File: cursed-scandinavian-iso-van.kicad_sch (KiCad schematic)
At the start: 105 parts, among them J1 Conn_01x04, SW1 SW_Push, U1 ATmega32U4-A, Y1 16MHz

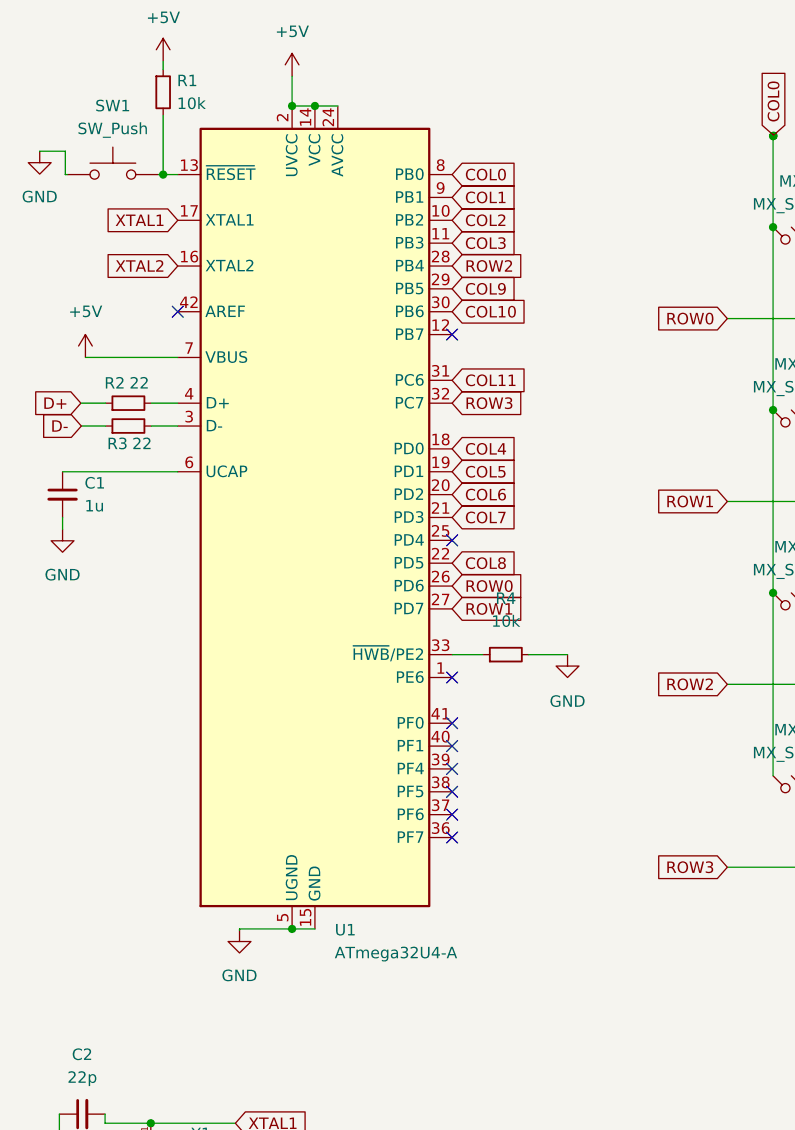
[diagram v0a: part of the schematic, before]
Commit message: second attempt
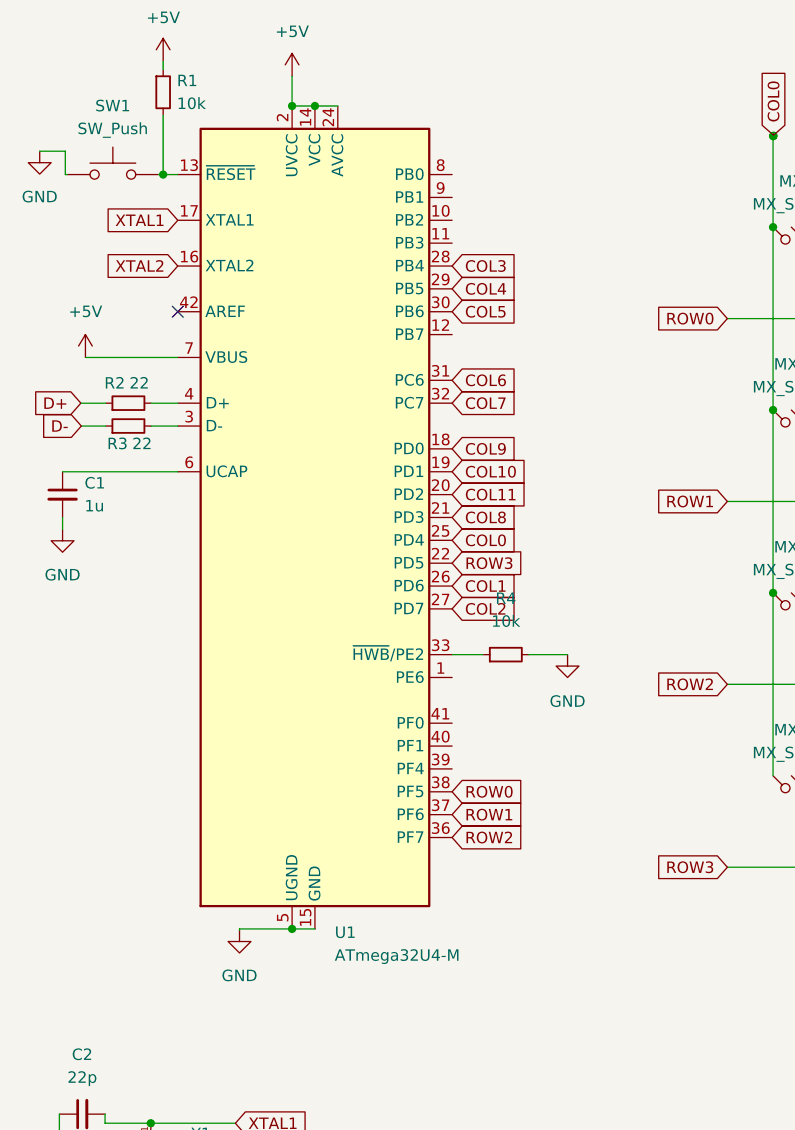
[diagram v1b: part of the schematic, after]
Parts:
- removed U1: ATmega32U4-A, Package_QFP:TQFP-44_10x10mm_P0.8mm, symbol MCU_Microchip_ATmega:ATmega32U4-A
- added U1: ATmega32U4-M, Package_DFN_QFN:QFN-44-1EP_7x7mm_P0.5mm_EP5.2x5.2mm, symbol MCU_Microchip_ATmega:ATmega32U4-M
- C1, C2, C3, C4, C5, C6, C7: footprint Capacitor_SMD:C_0805_2012Metric -> Capacitor_SMD:C_0402_1005Metric
- R1, R2, R3, R4: footprint Resistor_SMD:R_0805_2012Metric -> Resistor_SMD:R_0402_1005Metric
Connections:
- net +5V: now also U1.14 (VCC), U1.2 (UVCC), U1.24 (AVCC), U1.34 (VCC), U1.44 (AVCC), U1.7 (VBUS)
- net COL0: now also U1.25 (PD4)
- net COL1: now also U1.26 (PD6)
- net COL10: now also U1.19 (PD1)
- net COL11: now also U1.20 (PD2)
- net COL2: now also U1.27 (PD7)
- net COL3: now also U1.28 (PB4)
- net COL4: now also U1.29 (PB5)
- net COL5: now also U1.30 (PB6)
- net COL6: now also U1.31 (PC6)
- net COL7: now also U1.32 (PC7)
- net COL8: now also U1.21 (PD3)
- net COL9: now also U1.18 (PD0)
- net GND: now also U1.15 (GND), U1.23 (GND), U1.35 (GND), U1.43 (GND), U1.45 (GND), U1.5 (UGND)
- net ROW0: now also U1.38 (PF5)
- net ROW1: now also U1.37 (PF6)
- net ROW2: now also U1.36 (PF7)
- net ROW3: now also U1.22 (PD5)
- net XTAL1: now also U1.17 (XTAL1)
- net XTAL2: now also U1.16 (XTAL2)
- net at R1.2, SW1.1: now also U1.13 (~{RESET})
- net at R3.2: now also U1.3 (D-)
- net at R4.1: now also U1.33 (~{HWB}/PE2)
- net at R2.2: now also U1.4 (D+)
- net at C1.1: now also U1.6 (UCAP)
- no-connect marks 10 -> 1

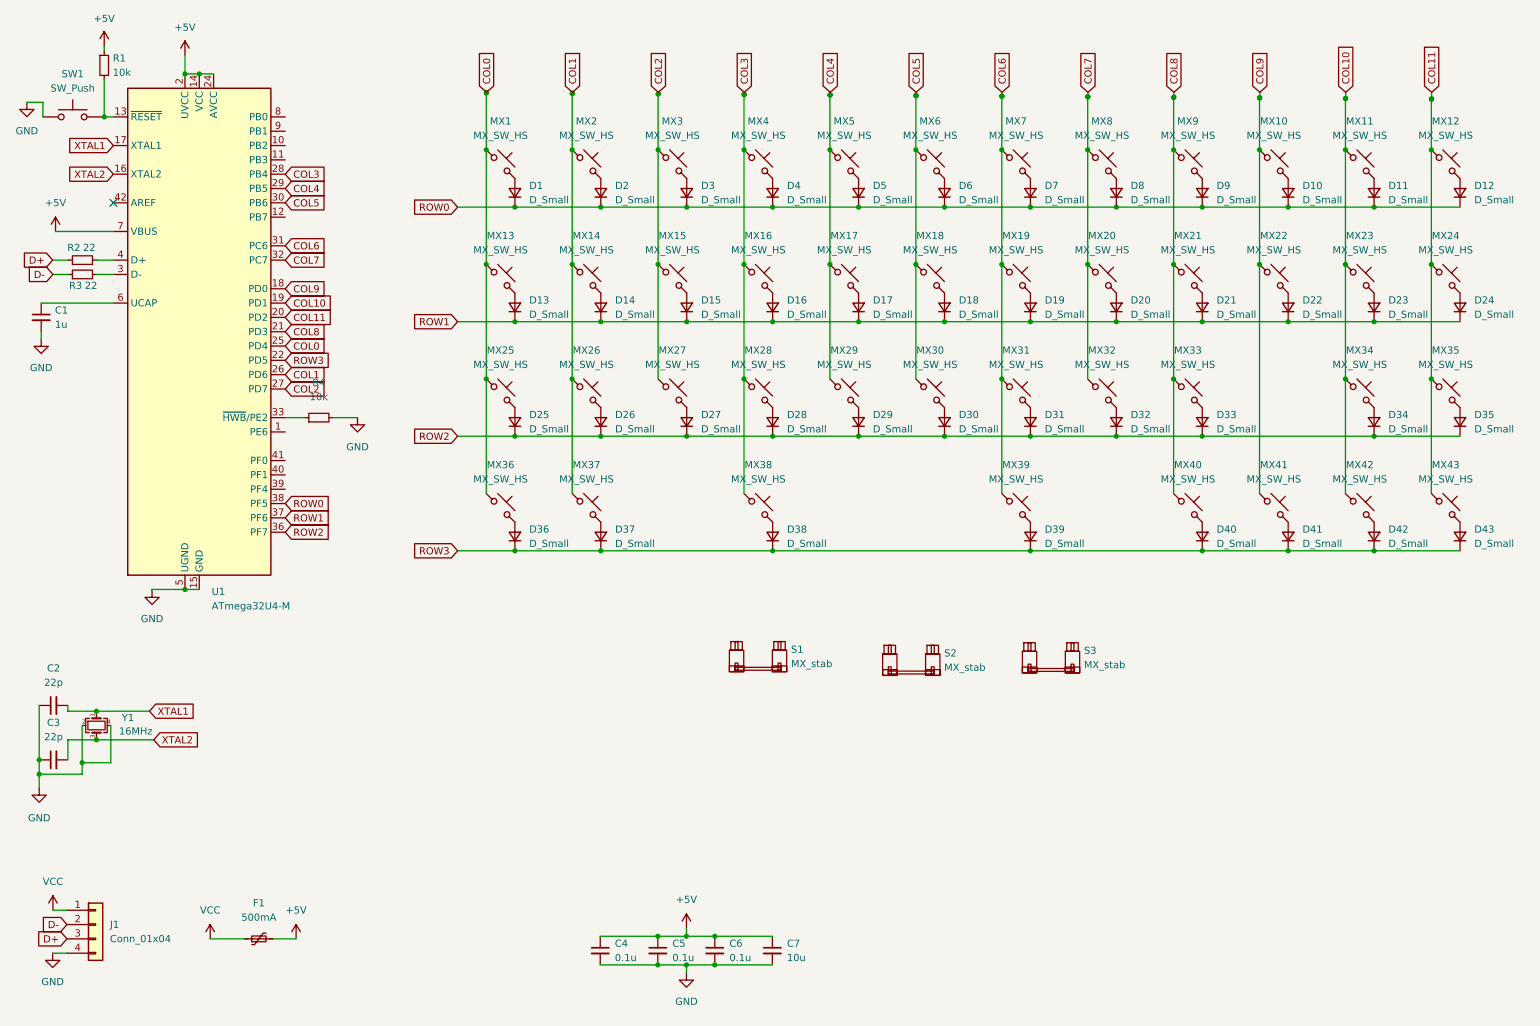
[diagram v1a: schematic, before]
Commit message: maybe
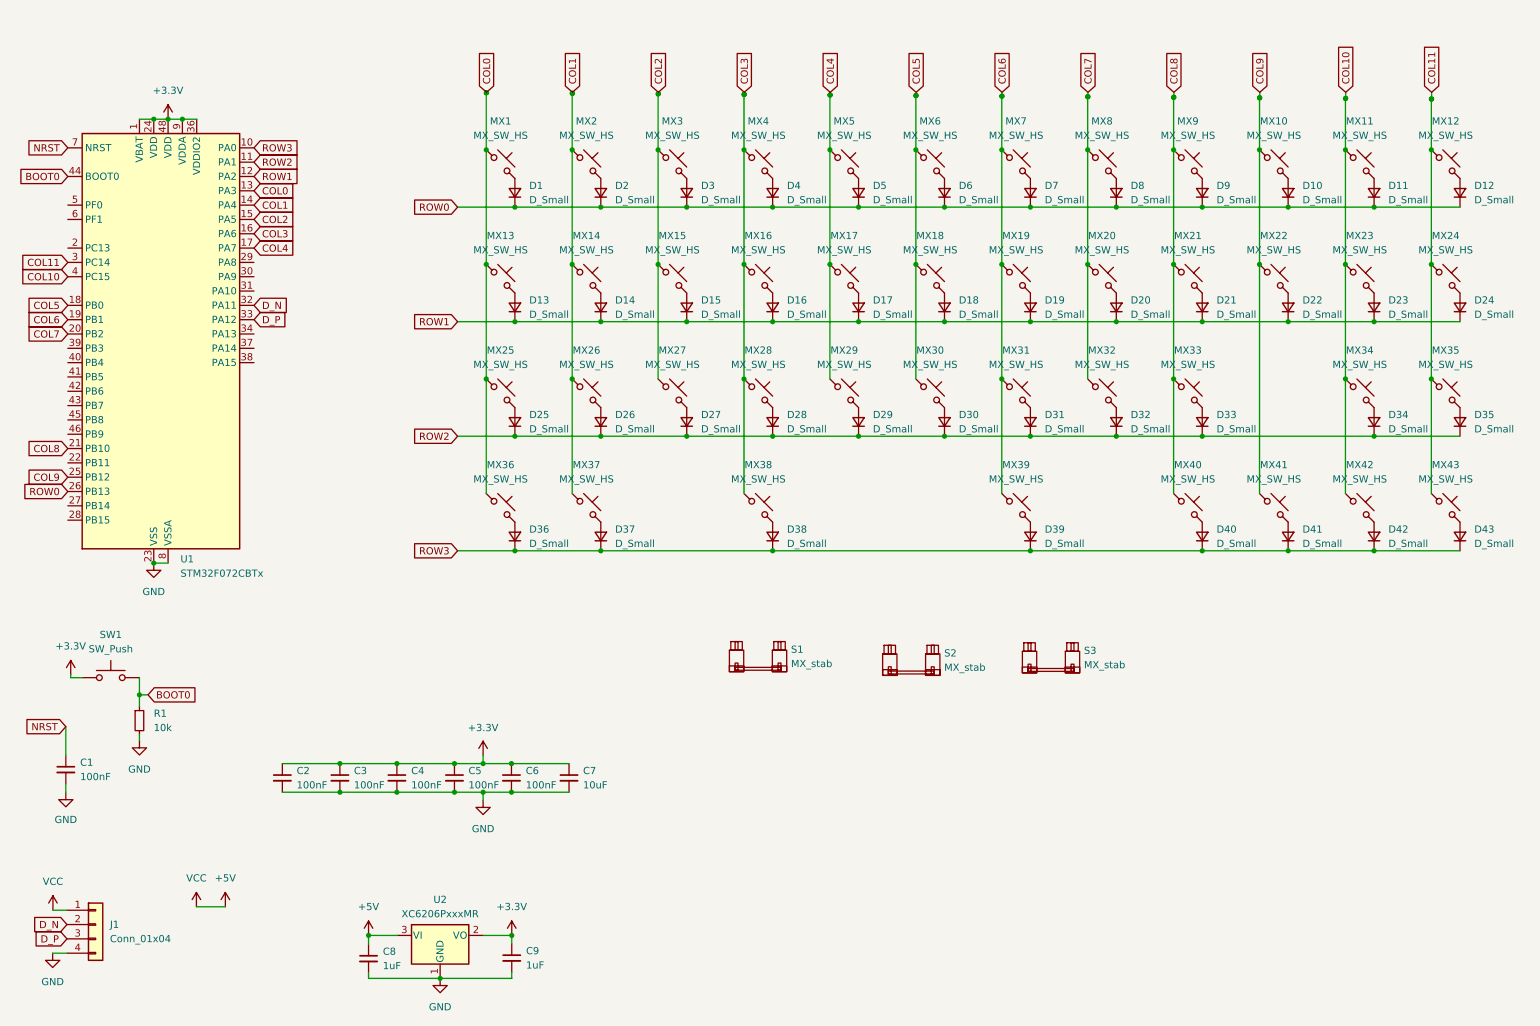
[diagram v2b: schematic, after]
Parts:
- removed F1: 500mA, Fuse:Fuse_1206_3216Metric, symbol Device:Polyfuse_Small
- removed R2, R3: 22, Resistor_SMD:R_0402_1005Metric, symbol Device:R_Small
- removed R4: 10k, Resistor_SMD:R_0402_1005Metric, symbol Device:R_Small
- removed U1: ATmega32U4-M, Package_DFN_QFN:QFN-44-1EP_7x7mm_P0.5mm_EP5.2x5.2mm, symbol MCU_Microchip_ATmega:ATmega32U4-M
- removed Y1: 16MHz, Crystal:Crystal_SMD_3225-4Pin_3.2x2.5mm, symbol Device:Crystal_GND24_Small
- added C8, C9: 1uF, Capacitor_SMD:C_0402_1005Metric, symbol Device:C_Small
- added U1: STM32F072CBTx, Package_QFP:LQFP-48_7x7mm_P0.5mm, symbol MCU_ST_STM32F0:STM32F072CBTx
- added U2: XC6206PxxxMR, Package_TO_SOT_SMD:SOT-23-3, symbol Regulator_Linear:XC6206PxxxMR
- C1: value 1u -> 100nF
- C2, C3: value 22p -> 100nF
- C4, C5, C6: value 0.1u -> 100nF
- C7: value 10u -> 10uF; footprint Capacitor_SMD:C_0402_1005Metric -> Capacitor_SMD:C_0603_1608Metric
- SW1: footprint Button_Switch_SMD:SW_SPST_TL3342 -> Button_Switch_SMD:SW_SPST_SKQG_WithoutStem
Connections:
- net VCC is gone; now on net +5V: J1.1 (Pin_1)
- net XTAL1 is gone; now on net GND: C2.2
- net XTAL2 is gone; now on net GND: C3.2
- net +5V: now also C8.1, U2.3 (VI); no longer C4.1, C5.1, C6.1, C7.1, R1.1
- net COL0: now also U1.13 (PA3)
- net COL1: now also U1.14 (PA4)
- net COL10: now also U1.4 (PC15)
- net COL11: now also U1.3 (PC14)
- net COL2: now also U1.15 (PA5)
- net COL3: now also U1.16 (PA6)
- net COL4: now also U1.17 (PA7)
- net COL5: now also U1.18 (PB0)
- net COL6: now also U1.19 (PB1)
- net COL7: now also U1.20 (PB2)
- net COL8: now also U1.21 (PB10)
- net COL9: now also U1.25 (PB12)
- net GND: now also R1.2, C8.2, C9.2, U1.23 (VSS), U1.35 (VSS), U1.47 (VSS), U1.8 (VSSA), U2.1 (GND); no longer C2.1, C3.1, SW1.2
- net ROW0: now also U1.26 (PB13)
- net ROW1: now also U1.12 (PA2)
- net ROW2: now also U1.11 (PA1)
- net ROW3: now also U1.10 (PA0)
- net +3.3V: now reaches SW1.1
- net +3.3V: now also C2.1, C3.1, C4.1, C5.1, C6.1, C7.1, C9.1, U1.1 (VBAT), U1.24 (VDD), U1.36 (VDDIO2), U1.48 (VDD), U1.9 (VDDA), U2.2 (VO); no longer R1.2
- net NRST: now reaches C1.1
- net NRST: now also U1.7 (NRST)
- net D+ renamed D_P
- net D_P: now also U1.33 (PA12)
- net D- renamed D_N
- net D_N: now also U1.32 (PA11)
- new net BOOT0: R1.1, SW1.2, U1.44 (BOOT0)
- no-connect marks 1 -> 0
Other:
- moved on the sheet: C4, C5, C6, C7
